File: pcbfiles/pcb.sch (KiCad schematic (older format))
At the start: 236 parts, among them J1 Conn_01x04_Female, J10 Conn_01x05, J2 Conn_01x05, J3 Conn_01x05, J4 Conn_01x05, J5 Conn_01x05, J6 Conn_01x04_Female, J7 Conn_01x05, J8 Conn_01x05, J9 Conn_01x05, Q1 AO3401A, Q2 AO3401A, SW1 SW_SPST, SW10 SW_SPST, SW11 SW_SPST, SW12 SW_SPST, SW13 SW_SPST, SW14 SW_SPST, SW15 SW_SPST, SW16 SW_SPST, SW17 SW_SPST, SW18 SW_SPST, SW19 SW_SPST, SW2 SW_SPST, SW20 SW_SPST, SW21 SW_SPST, SW22 SW_SPST, SW23 SW_SPST, SW24 SW_SPST, SW25 SW_SPST, SW26 SW_SPST, SW27 SW_SPST, SW28 SW_SPST, SW29 SW_SPST, SW3 SW_SPST, SW30 SW_SPST, SW31 SW_SPST, SW32 SW_SPST, SW33 SW_SPST, SW34 SW_SPST, SW35 SW_SPST, SW36 SW_SPST, SW37 SW_SPST, SW38 SW_SPDT, SW39 SW_SPST, SW4 SW_SPST, SW40 SW_SPST, SW41 SW_SPST, SW42 SW_SPST, SW43 SW_SPST, SW44 SW_SPST, SW45 SW_SPST, SW46 Rotary_Encoder_Switch, SW47 SW_SPDT, SW48 SW_SPST, SW49 SW_SPST, SW5 SW_SPST, SW50 SW_SPST, SW51 SW_SPST, SW52 SW_SPST, SW53 SW_SPST, SW54 SW_SPST, SW55 SW_SPST, SW56 SW_SPST, SW57 SW_SPST, SW58 SW_SPST, SW59 SW_SPST, SW6 SW_SPST, SW60 SW_SPST, SW61 SW_SPST, SW62 SW_SPST, SW63 SW_SPST, SW64 SW_SPST, SW65 SW_SPST, SW66 SW_SPST, SW67 SW_SPST, SW68 SW_SPST, SW69 SW_SPST, SW7 SW_SPST, SW70 SW_SPST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

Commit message: remove JST for thumb keys and move batt connector
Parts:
- removed J3, J7, J8: Conn_01x05, Connector_JST:JST_SH_SM05B-SRSS-TB_1x05-1MP_P1.00mm_Horizontal, symbol Connector_Generic:Conn_01x05
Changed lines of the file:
@@
 Wire Wire Line
 	9200 4450 8500 4450
-$Comp
-L Connector_Generic:Conn_01x05 J2
-U 1 1 612FA838
-P 6250 7050
-F 0 "J2" V 6214 6762 50  0000 R CNN
-F 1 "Conn_01x05" V 6123 6762 50  0000 R CNN
-F 2 "Connector_JST:JST_SH_SM05B-SRSS-TB_1x05-1MP_P1.00mm_Horizontal" H 6250 7050 50  0001 C CNN
-F 3 "~" H 6250 7050 50  0001 C CNN
-	1    6250 7050
-	0    -1   -1   0
-$EndComp
 Text GLabel 6150 7250 3    50   Input ~ 0
 DB1_COL0
@@
 F 3 "~" V 9150 8550 50  0001 C CNN
 	1    9150 8550
-	0    -1   -1   0
-$EndComp
-$Comp
-L Connector_Generic:Conn_01x05 J3
-U 1 1 615D7014
-P 6950 7050
-F 0 "J3" V 6914 6762 50  0000 R CNN
-F 1 "Conn_01x05" V 6823 6762 50  0000 R CNN
-F 2 "Connector_JST:JST_SH_SM05B-SRSS-TB_1x05-1MP_P1.00mm_Horizontal" H 6950 7050 50  0001 C CNN
-F 3 "~" H 6950 7050 50  0001 C CNN
-	1    6950 7050
 	0    -1   -1   0
 $EndComp
@@
 Wire Wire Line
 	25800 3900 25100 3900
-$Comp
-L Connector_Generic:Conn_01x05 J7
-U 1 1 6175E909
-P 22450 6500
-F 0 "J7" V 22414 6212 50  0000 R CNN
-F 1 "Conn_01x05" V 22323 6212 50  0000 R CNN
-F 2 "Connector_JST:JST_SH_SM05B-SRSS-TB_1x05-1MP_P1.00mm_Horizontal" H 22450 6500 50  0001 C CNN
-F 3 "~" H 22450 6500 50  0001 C CNN
-	1    22450 6500
-	0    -1   -1   0
-$EndComp
 Text GLabel 22350 6700 3    50   Input ~ 0
 DB1_COL0_B
@@
 $EndComp
 $Comp
-L Connector_Generic:Conn_01x05 J8
-U 1 1 6175E9B4
-P 23150 6500
-F 0 "J8" V 23114 6212 50  0000 R CNN
-F 1 "Conn_01x05" V 23023 6212 50  0000 R CNN
-F 2 "Connector_JST:JST_SH_SM05B-SRSS-TB_1x05-1MP_P1.00mm_Horizontal" H 23150 6500 50  0001 C CNN
-F 3 "~" H 23150 6500 50  0001 C CNN
-	1    23150 6500
-	0    -1   -1   0
-$EndComp
-$Comp
 L power:GND1 #PWR0131
 U 1 1 6175E9BE
@@
 	1    0    0    -1
 $EndComp
-$Comp
-L Connector_Generic:Conn_01x05 J9
-U 1 1 6175E9CA
-P 25650 6500
-F 0 "J9" V 25614 6212 50  0000 R CNN
-F 1 "Conn_01x05" V 25523 6212 50  0000 R CNN
-F 2 "Connector_JST:JST_SH_SM05B-SRSS-TB_1x05-1MP_P1.00mm_Horizontal" H 25650 6500 50  0001 C CNN
-F 3 "~" H 25650 6500 50  0001 C CNN
-	1    25650 6500
-	0    -1   -1   0
-$EndComp
 Text GLabel 25450 6700 3    50   Input ~ 0
 DB2_COL0_B
@@
 	1    25850 6700
 	1    0    0    -1
-$EndComp
-$Comp
-L Connector_Generic:Conn_01x05 J10
-U 1 1 6175E9DA
-P 26350 6500
-F 0 "J10" V 26314 6212 50  0000 R CNN
-F 1 "Conn_01x05" V 26223 6212 50  0000 R CNN
-F 2 "Connector_JST:JST_SH_SM05B-SRSS-TB_1x05-1MP_P1.00mm_Horizontal" H 26350 6500 50  0001 C CNN
-F 3 "~" H 26350 6500 50  0001 C CNN
-	1    26350 6500
-	0    -1   -1   0
 $EndComp
 Text GLabel 26150 6700 3    50   Input ~ 0
@@
 Text GLabel 16900 5400 0    50   Input ~ 0
 DB2_COL2_B
+$Comp
+L Connector_Generic:Conn_01x05 J10
+U 1 1 6175E9DA
+P 26350 6500
+F 0 "J10" V 26314 6212 50  0000 R CNN
+F 1 "Conn_01x05" V 26223 6212 50  0000 R CNN
+F 2 "Connector_JST:JST_SH_SM05B-SRSS-TB_1x05-1MP_P1.00mm_Horizontal" H 26350 6500 50  0001 C CNN
+F 3 "~" H 26350 6500 50  0001 C CNN
+	1    26350 6500
+	0    -1   -1   0
+$EndComp
+$Comp
+L Connector_Generic:Conn_01x05 J9
+U 1 1 6175E9CA
+P 25650 6500
+F 0 "J9" V 25614 6212 50  0000 R CNN
+F 1 "Conn_01x05" V 25523 6212 50  0000 R CNN
+F 2 "Connector_JST:JST_SH_SM05B-SRSS-TB_1x05-1MP_P1.00mm_Horizontal" H 25650 6500 50  0001 C CNN
+F 3 "~" H 25650 6500 50  0001 C CNN
+	1    25650 6500
+	0    -1   -1   0
+$EndComp
+$Comp
+L Connector_Generic:Conn_01x05 J2
+U 1 1 612FA838
+P 6250 7050
+F 0 "J2" V 6214 6762 50  0000 R CNN
+F 1 "Conn_01x05" V 6123 6762 50  0000 R CNN
+F 2 "Connector_JST:JST_SH_SM05B-SRSS-TB_1x05-1MP_P1.00mm_Horizontal" H 6250 7050 50  0001 C CNN
+F 3 "~" H 6250 7050 50  0001 C CNN
+	1    6250 7050
+	0    -1   -1   0
+$EndComp
 $EndSCHEMATC

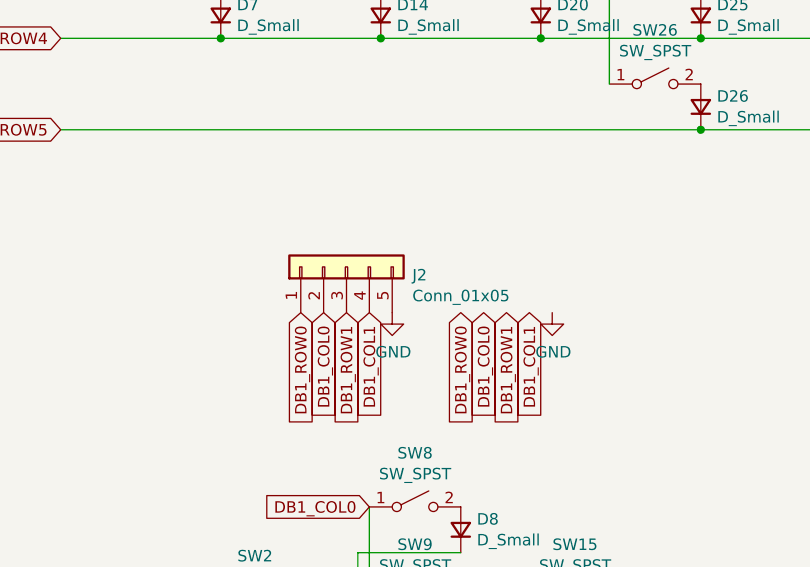
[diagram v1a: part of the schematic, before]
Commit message: minor changes, production files
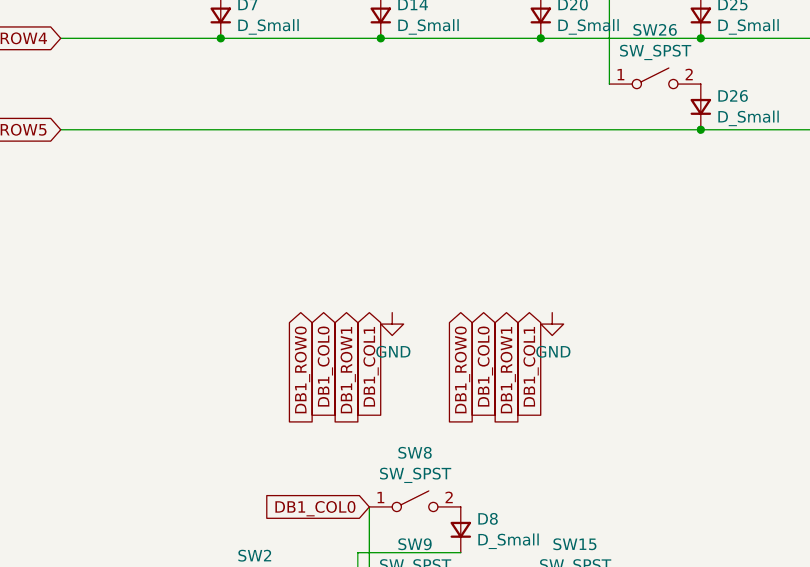
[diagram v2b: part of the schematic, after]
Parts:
- removed J2: Conn_01x05, Connector_JST:JST_SH_SM05B-SRSS-TB_1x05-1MP_P1.00mm_Horizontal, symbol Connector_Generic:Conn_01x05
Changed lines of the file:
@@
-	0    -1   -1   0
-$EndComp
-$Comp
-L Connector_Generic:Conn_01x05 J2
-U 1 1 612FA838
-P 6250 7050
-F 0 "J2" V 6214 6762 50  0000 R CNN
-F 1 "Conn_01x05" V 6123 6762 50  0000 R CNN
-F 2 "Connector_JST:JST_SH_SM05B-SRSS-TB_1x05-1MP_P1.00mm_Horizontal" H 6250 7050 50  0001 C CNN
-F 3 "~" H 6250 7050 50  0001 C CNN
-	1    6250 7050
 	0    -1   -1   0
 $EndComp
